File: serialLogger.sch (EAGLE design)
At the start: 35 parts, among them J1 Ext Pwr, U1 MCP1702, U2 MCP1700, U3 ATmega328P-AU, U4 74HC4050PW, X1 MICROSD, Y1 16MHz

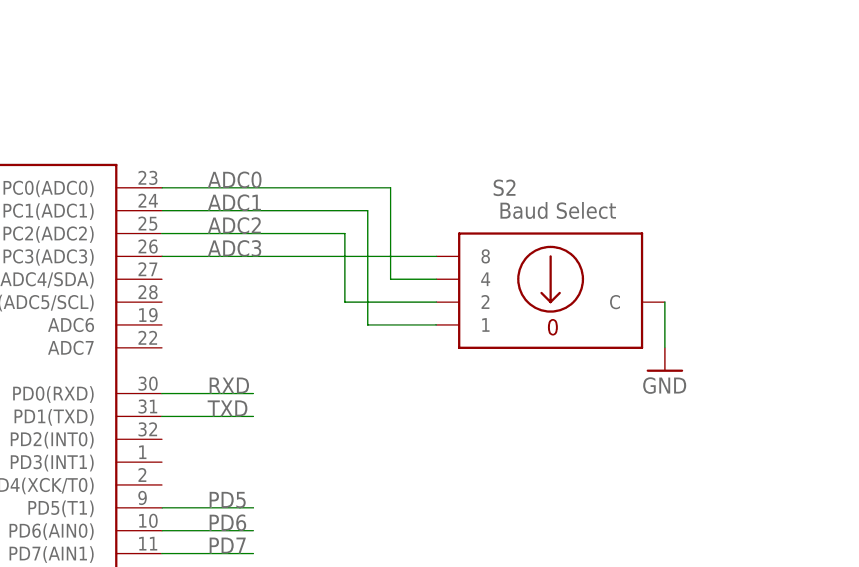
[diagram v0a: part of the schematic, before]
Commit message: Final v2 board
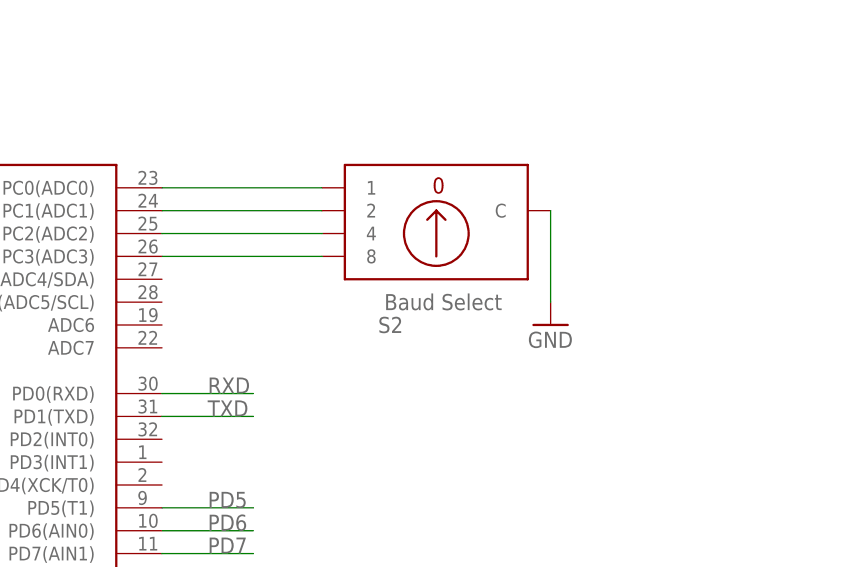
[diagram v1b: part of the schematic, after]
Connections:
- net ADC3 renamed N$8
- removed net ADC0: S2.4, U3.PC0(ADC0)
- removed net ADC1: S2.1, U3.PC1(ADC1)
- removed net ADC2: S2.2, U3.PC2(ADC2)
- new net N$5: S2.1, U3.PC0(ADC0)
- new net N$6: S2.2, U3.PC1(ADC1)
- new net N$7: S2.4, U3.PC2(ADC2)
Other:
- moved on the sheet: S2
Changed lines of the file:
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@@
 <attribute name="VALUE" x="51.308" y="59.69" size="1.778" layer="96"/>
 </instance>
-<instance part="S2" gate="G$1" x="226.06" y="121.92" smashed="yes">
-<attribute name="NAME" x="220.98" y="132.08" size="1.778" layer="95" align="center"/>
-<attribute name="VALUE" x="226.822" y="129.54" size="1.778" layer="96" align="center"/>
+<instance part="S2" gate="G$1" x="213.36" y="127" smashed="yes" rot="MR180">
+<attribute name="NAME" x="208.28" y="116.84" size="1.778" layer="95" rot="MR180" align="center"/>
+<attribute name="VALUE" x="214.122" y="119.38" size="1.778" layer="96" rot="MR180" align="center"/>
 </instance>
-<instance part="GND4" gate="1" x="238.76" y="111.76"/>
+<instance part="GND4" gate="1" x="226.06" y="116.84"/>
 <instance part="+3V1" gate="G$1" x="63.5" y="114.3" smashed="yes">
 <attribute name="VALUE" x="61.468" y="115.57" size="1.778" layer="96"/>
@@
 <pinref part="S2" gate="G$1" pin="C"/>
 <pinref part="GND4" gate="1" pin="GND"/>
-<wire x1="238.76" y1="119.38" x2="238.76" y2="114.3" width="0.1524" layer="91"/>
+<wire x1="226.06" y1="129.54" x2="226.06" y2="119.38" width="0.1524" layer="91"/>
 </segment>
 <segment>
@@
 </segment>
 </net>
-<net name="ADC3" class="0">
-<segment>
-<pinref part="U3" gate="G$1" pin="PC3(ADC3)"/>
-<wire x1="182.88" y1="124.46" x2="213.36" y2="124.46" width="0.1524" layer="91"/>
-<label x="187.96" y="124.46" size="1.778" layer="95"/>
-<pinref part="S2" gate="G$1" pin="8"/>
-</segment>
-</net>
-<net name="ADC2" class="0">
-<segment>
-<pinref part="U3" gate="G$1" pin="PC2(ADC2)"/>
-<label x="187.96" y="127" size="1.778" layer="95"/>
-<pinref part="S2" gate="G$1" pin="2"/>
-<wire x1="213.36" y1="119.38" x2="203.2" y2="119.38" width="0.1524" layer="91"/>
-<wire x1="203.2" y1="119.38" x2="203.2" y2="127" width="0.1524" layer="91"/>
-<wire x1="203.2" y1="127" x2="182.88" y2="127" width="0.1524" layer="91"/>
-</segment>
-</net>
-<net name="ADC1" class="0">
-<segment>
-<pinref part="U3" gate="G$1" pin="PC1(ADC1)"/>
-<wire x1="182.88" y1="129.54" x2="205.74" y2="129.54" width="0.1524" layer="91"/>
-<label x="187.96" y="129.54" size="1.778" layer="95"/>
-<pinref part="S2" gate="G$1" pin="1"/>
-<wire x1="213.36" y1="116.84" x2="205.74" y2="116.84" width="0.1524" layer="91"/>
-<wire x1="205.74" y1="116.84" x2="205.74" y2="129.54" width="0.1524" layer="91"/>
-</segment>
-</net>
-<net name="ADC0" class="0">
-<segment>
-<pinref part="U3" gate="G$1" pin="PC0(ADC0)"/>
-<wire x1="182.88" y1="132.08" x2="208.28" y2="132.08" width="0.1524" layer="91"/>
-<label x="187.96" y="132.08" size="1.778" layer="95"/>
-<pinref part="S2" gate="G$1" pin="4"/>
-<wire x1="213.36" y1="121.92" x2="208.28" y2="121.92" width="0.1524" layer="91"/>
-<wire x1="208.28" y1="121.92" x2="208.28" y2="132.08" width="0.1524" layer="91"/>
-</segment>
-</net>
 <net name="/SS" class="0">
 <segment>
@@
 </segment>
 </net>
+<net name="N$5" class="0">
+<segment>
+<pinref part="S2" gate="G$1" pin="1"/>
+<pinref part="U3" gate="G$1" pin="PC0(ADC0)"/>
+<wire x1="200.66" y1="132.08" x2="182.88" y2="132.08" width="0.1524" layer="91"/>
+</segment>
+</net>
+<net name="N$6" class="0">
+<segment>
+<pinref part="S2" gate="G$1" pin="2"/>
+<pinref part="U3" gate="G$1" pin="PC1(ADC1)"/>
+<wire x1="200.66" y1="129.54" x2="182.88" y2="129.54" width="0.1524" layer="91"/>
+</segment>
+</net>
+<net name="N$7" class="0">
+<segment>
+<pinref part="S2" gate="G$1" pin="4"/>
+<pinref part="U3" gate="G$1" pin="PC2(ADC2)"/>
+<wire x1="200.66" y1="127" x2="182.88" y2="127" width="0.1524" layer="91"/>
+</segment>
+</net>
+<net name="N$8" class="0">
+<segment>
+<pinref part="S2" gate="G$1" pin="8"/>
+<pinref part="U3" gate="G$1" pin="PC3(ADC3)"/>
+<wire x1="200.66" y1="124.46" x2="182.88" y2="124.46" width="0.1524" layer="91"/>
+</segment>
+</net>
